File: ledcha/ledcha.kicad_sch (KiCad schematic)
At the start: 18 parts, among them J1 Conn_01x02, U1 NE555P, U2 4017

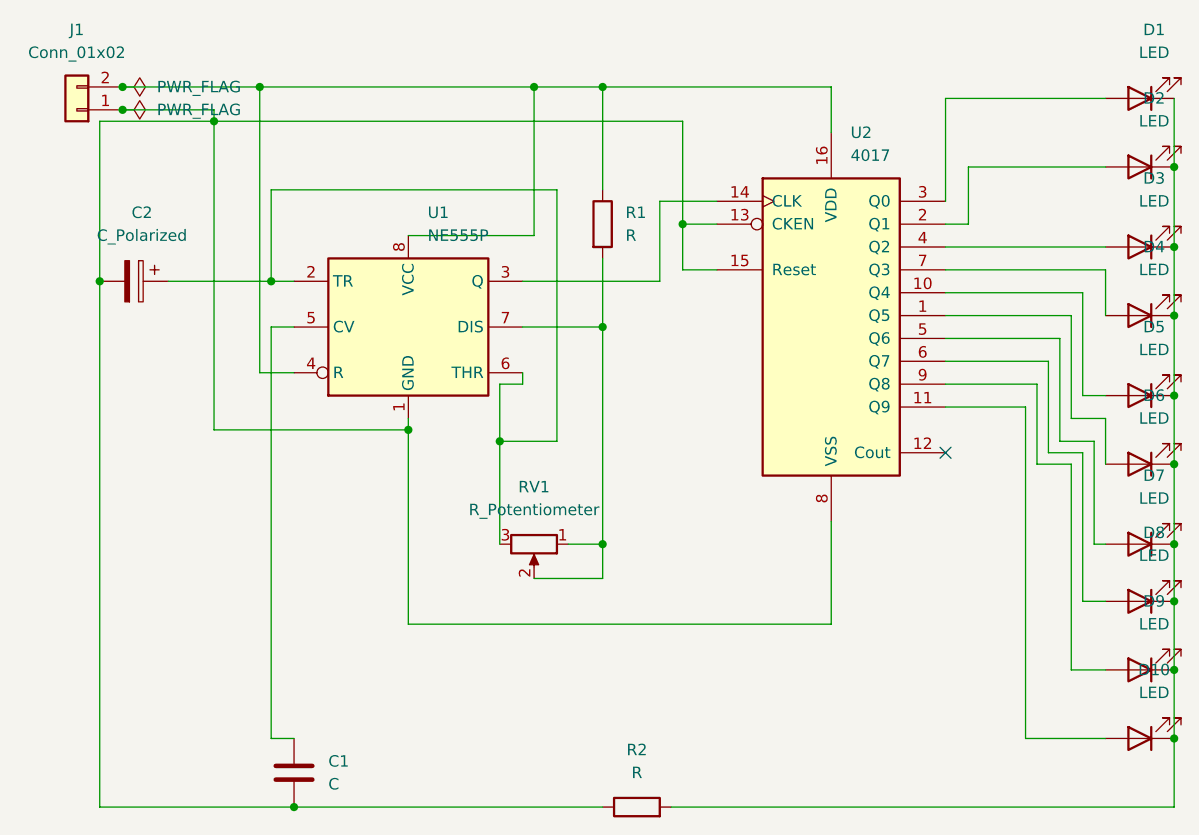
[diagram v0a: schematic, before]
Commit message: uploaded all files
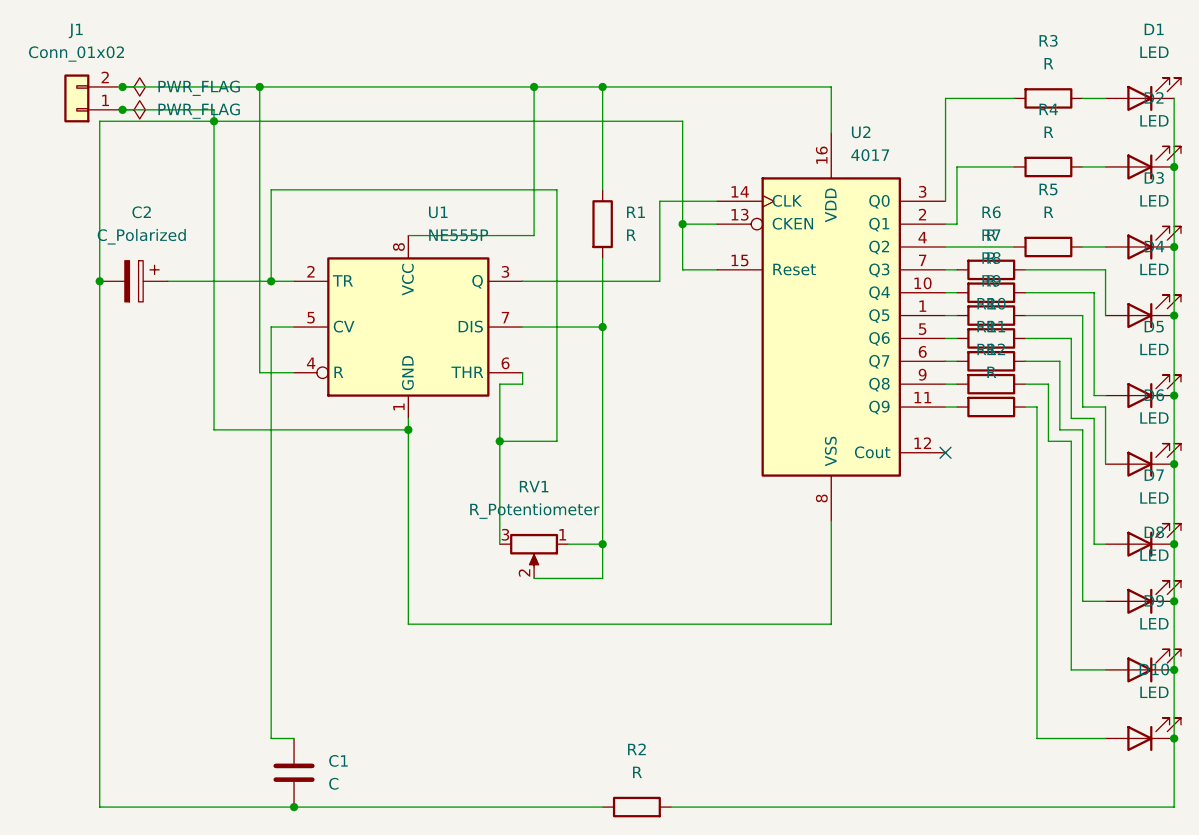
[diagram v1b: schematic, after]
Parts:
- added R10, R11, R12, R3, R4, R5, R6, R7, R8, R9: R, Resistor_THT:R_Axial_DIN0207_L6.3mm_D2.5mm_P7.62mm_Horizontal, symbol Device:R
- D2: footprint Connector_PinHeader_2.54mm:PinHeader_1x02_P2.54mm_Vertical -> LED_THT:LED_D5.0mm
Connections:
- net at D6.2 (A): now also R8.1; no longer U2.1 (Q5)
- net at D2.2 (A): now also R4.1; no longer U2.2 (Q1)
- net at D5.2 (A): now also R7.1; no longer U2.10 (Q4)
- net at D3.2 (A): now also R5.1; no longer U2.4 (Q2)
- net at D4.2 (A): now also R6.1; no longer U2.7 (Q3)
- net at D8.2 (A): now also R10.1; no longer U2.6 (Q7)
- net at D7.2 (A): now also R9.1; no longer U2.5 (Q6)
- net at D10.2 (A): now also R12.1; no longer U2.11 (Q9)
- net at D9.2 (A): now also R11.1; no longer U2.9 (Q8)
- net at D1.2 (A): now also R3.1; no longer U2.3 (Q0)
- new net: R12.2, U2.11 (Q9)
- new net: R3.2, U2.3 (Q0)
- new net: R11.2, U2.9 (Q8)
- new net: R4.2, U2.2 (Q1)
- new net: R6.2, U2.7 (Q3)
- new net: R10.2, U2.6 (Q7)
- new net: R5.2, U2.4 (Q2)
- new net: R7.2, U2.10 (Q4)
- new net: R8.2, U2.1 (Q5)
- new net: R9.2, U2.5 (Q6)
